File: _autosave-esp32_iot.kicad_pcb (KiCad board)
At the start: 4 copper layers, 134 x 63.8 mm, 84 parts, among them J1 B2B-PH-SM4-TB, J2 SS-52400-002, J3 GSD090012SEU, J4 Conn_01x04_Pin, J5 Conn_01x05_Pin, Q1 BC817, Q2 TEMT6000X01, Q3 BC817, U1 MCP73871, U2 USBLC6-2SC6, U3 CP2102N-Axx-xQFN20, U4 W25Q32JVSSIQ, U5 ESP32-C3-WROOM-02-H4, U6 BME280, U7 MAX4466EXK

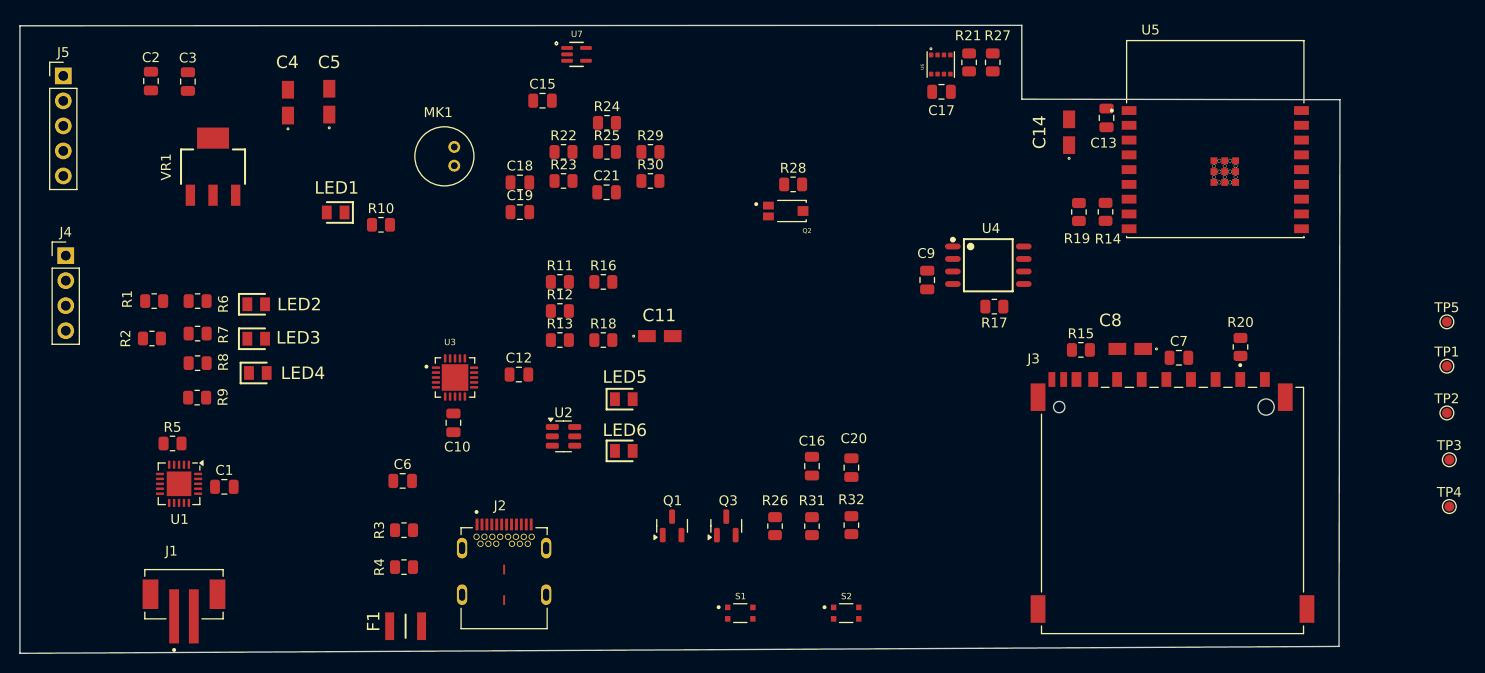
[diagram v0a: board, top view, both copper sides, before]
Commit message: placement complete
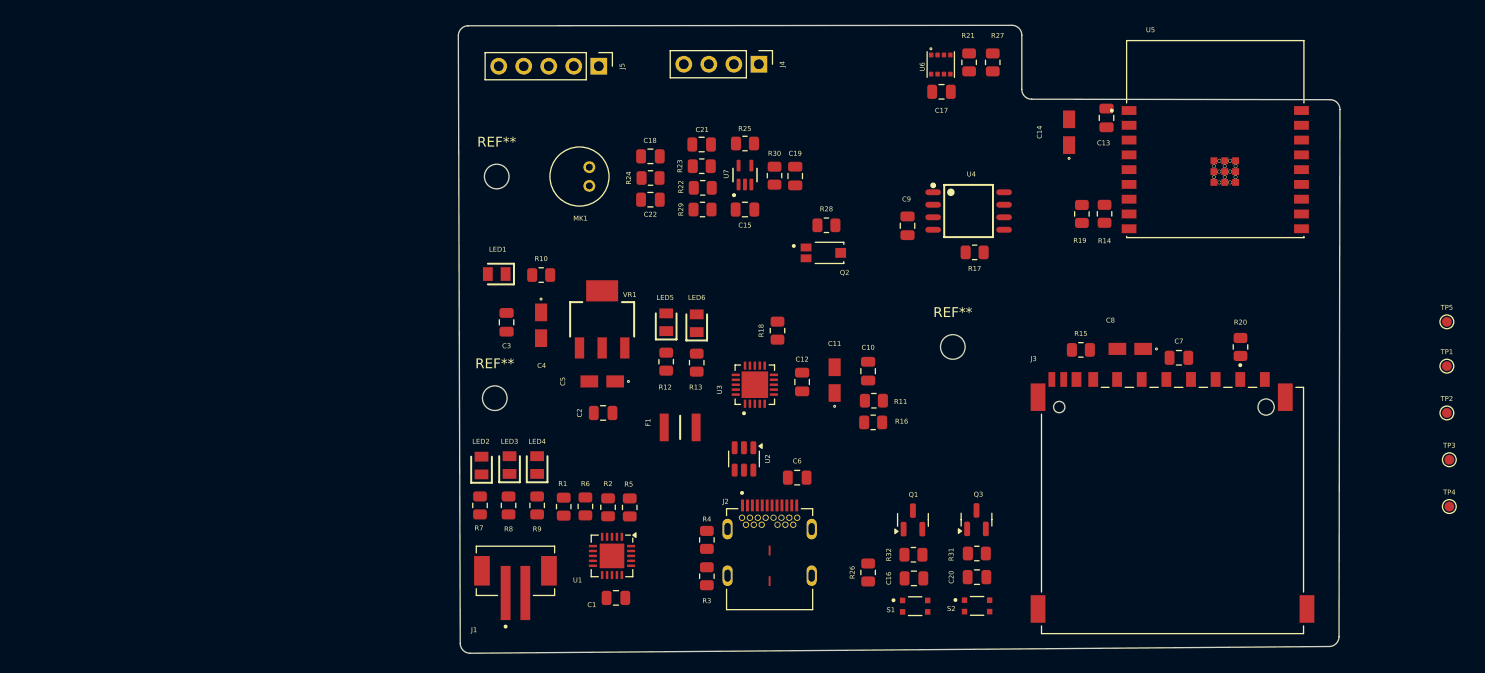
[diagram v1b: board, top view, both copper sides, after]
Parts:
- added C22: 10n, Capacitor_SMD:C_0805_2012Metric, F.Cu at (133.1, 78.5)
- added REF**: MountingHole_2.5mm, MountingHole:MountingHole_2.5mm, F.Cu at (117.3, 98.6)
- added REF**: MountingHole_2.5mm, MountingHole:MountingHole_2.5mm, F.Cu at (117.5, 76.1)
- added REF**: MountingHole_2.5mm, MountingHole:MountingHole_2.5mm, F.Cu at (163.8, 93.4)
- moved J4 73.0 mm to (144.1, 64.7), turned to -90 degrees
- moved C2 56.9 mm to (128.3, 100.1), turned to 180 degrees
- moved J5 54.4 mm to (127.9, 64.9), turned to -90 degrees
- moved R2 49.4 mm to (128.8, 109.7), turned to 90 degrees
- moved R5 46.9 mm to (131.0, 109.7), turned to -90 degrees
- moved R1 46.5 mm to (124.3, 109.6), turned to 90 degrees
- moved U1 44.6 mm to (129.2, 114.6)
- moved R6 44.5 mm to (126.5, 109.6), turned to -90 degrees
- moved VR1 42.4 mm to (128.2, 90.6)
- moved C10 42.4 mm to (155.2, 95.9)
- moved C1 41.3 mm to (129.6, 118.9)
- moved C3 40.5 mm to (118.5, 90.9), turned to -90 degrees
- moved C6 40.1 mm to (148.0, 106.7)
- moved C5 39.7 mm to (128.2, 96.9), turned to 180 degrees
- moved R9 36.2 mm to (121.6, 109.5), turned to 90 degrees
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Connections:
- MK1 pad OUT: Net-(U7-IN+) -> Net-(C22-Pad1)
- R24 pad 2: Net-(U7-IN+) -> Net-(C22-Pad1)
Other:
- board size 134 x 63.8 mm -> 89.5 x 63.7 mm
